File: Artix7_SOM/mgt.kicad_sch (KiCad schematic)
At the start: 1 part, among them U1 XC7A100T-FGG676

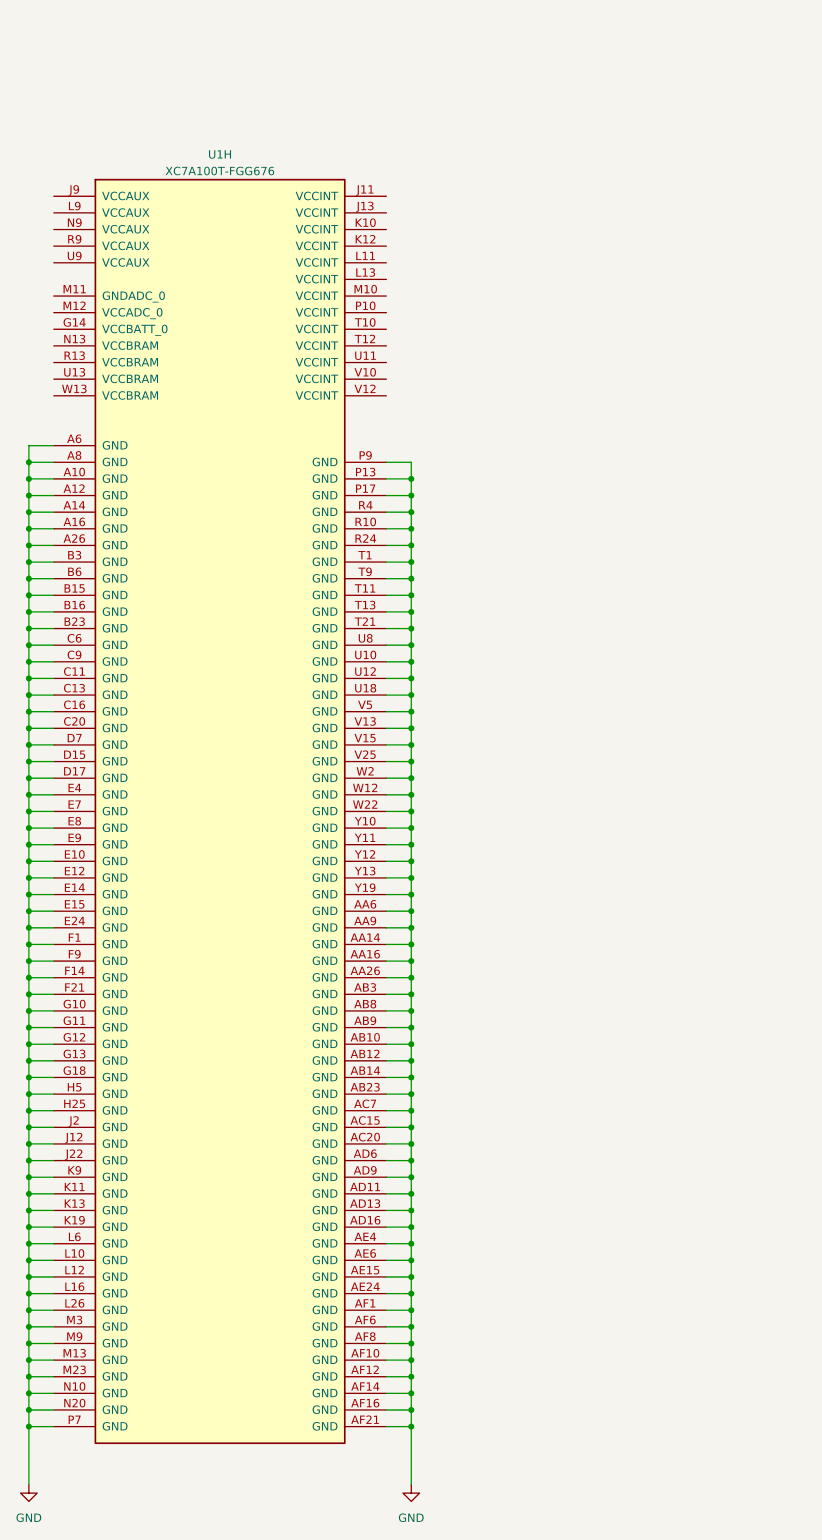
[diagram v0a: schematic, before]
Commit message: update
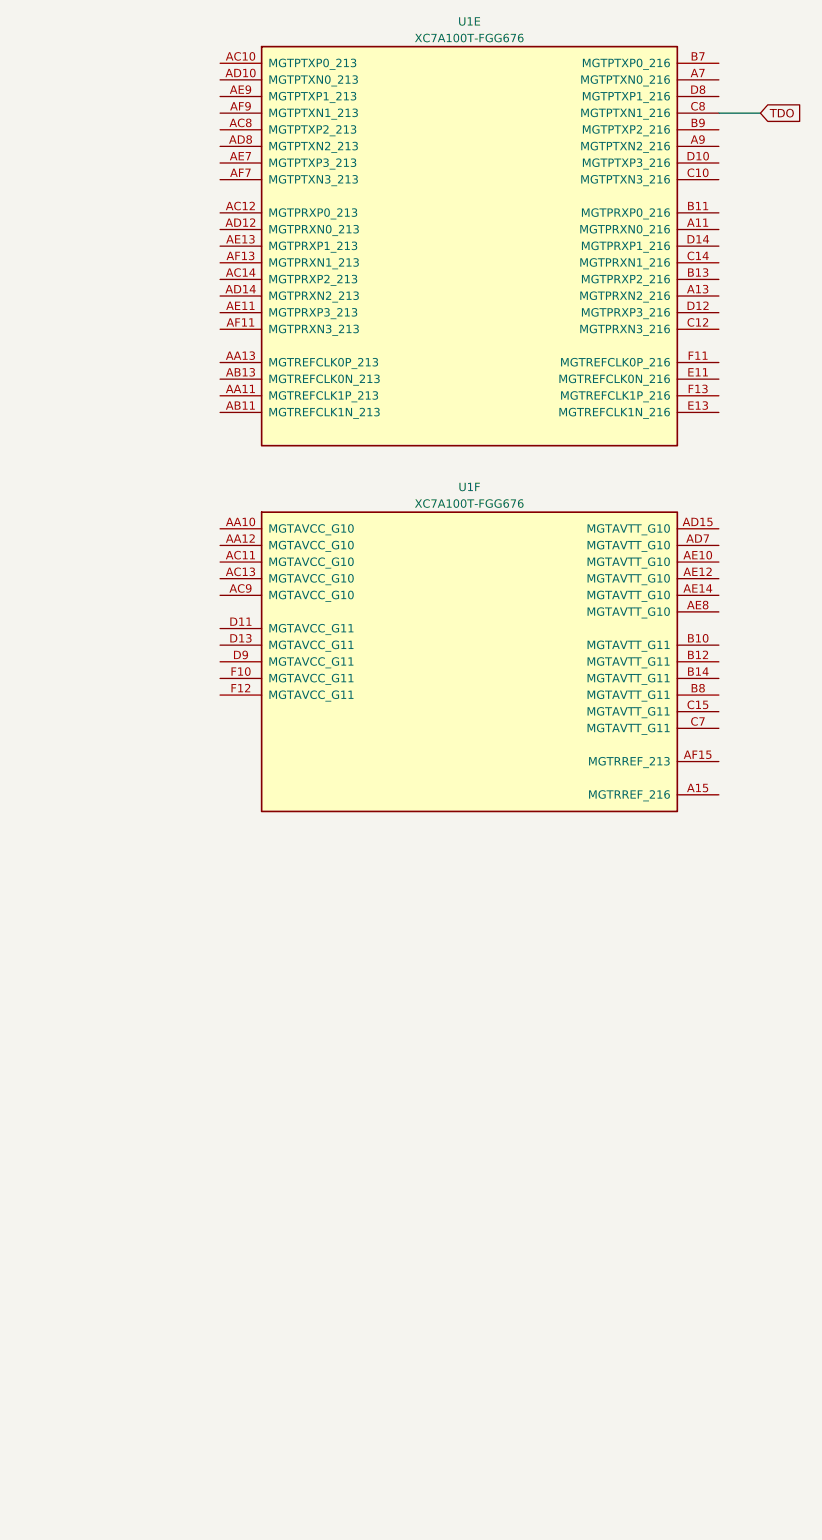
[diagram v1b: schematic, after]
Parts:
- removed U1: XC7A100T-FGG676, Package_BGA:Xilinx_FGG676, symbol FPGA_Xilinx_Artix7:XC7A100T-FGG676
- added U1: XC7A100T-FGG676, Package_BGA:Xilinx_FGG676, symbol FPGA_Xilinx_Artix7:XC7A100T-FGG676
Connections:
- new net TDO: U1.C8 (MGTPTXN1_216)
